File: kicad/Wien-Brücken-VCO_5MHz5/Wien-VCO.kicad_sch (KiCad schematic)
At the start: 22 parts, among them J1 J113, U1 ${SIM.NAME}

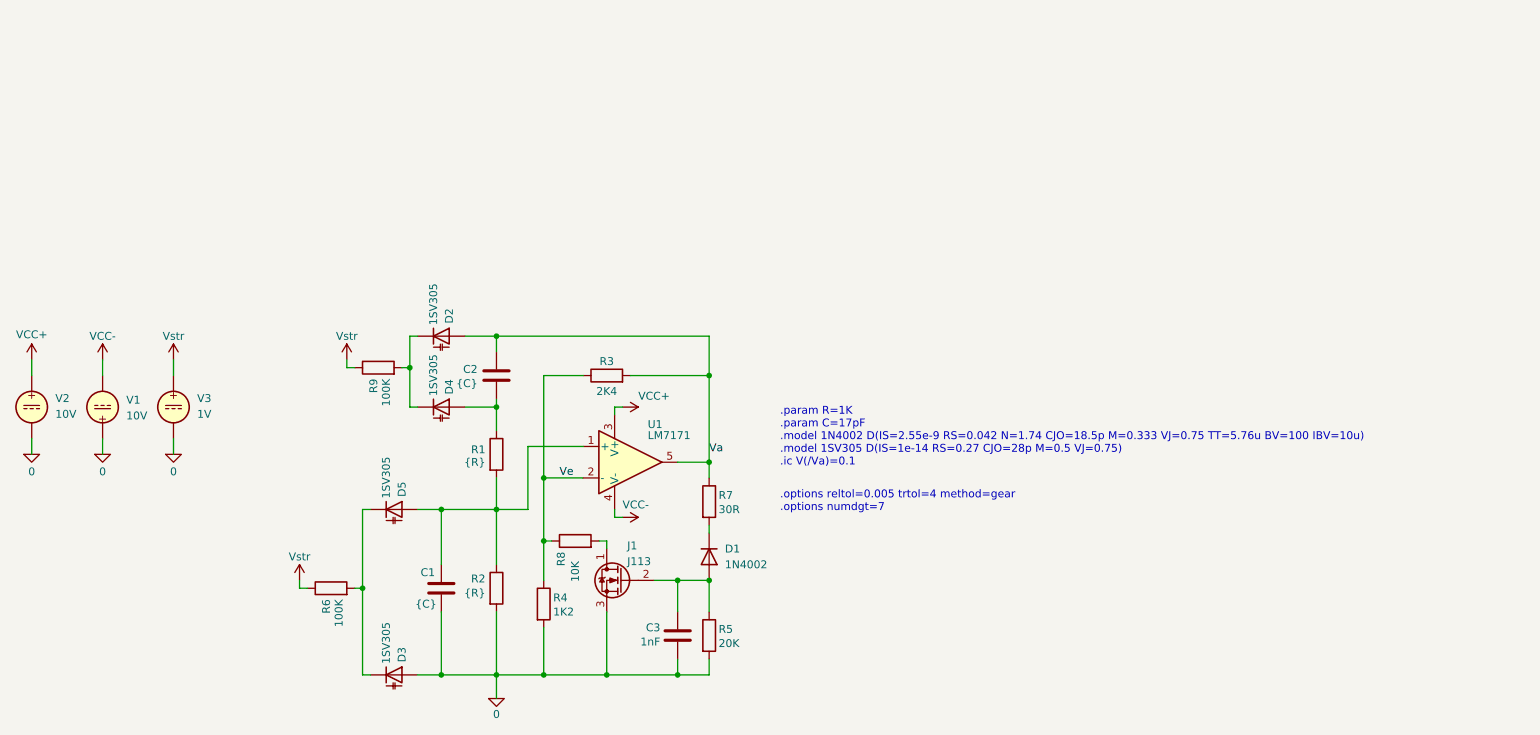
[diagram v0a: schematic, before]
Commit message: Erste Änderungen, Abgleiche LTspice vs ngspice
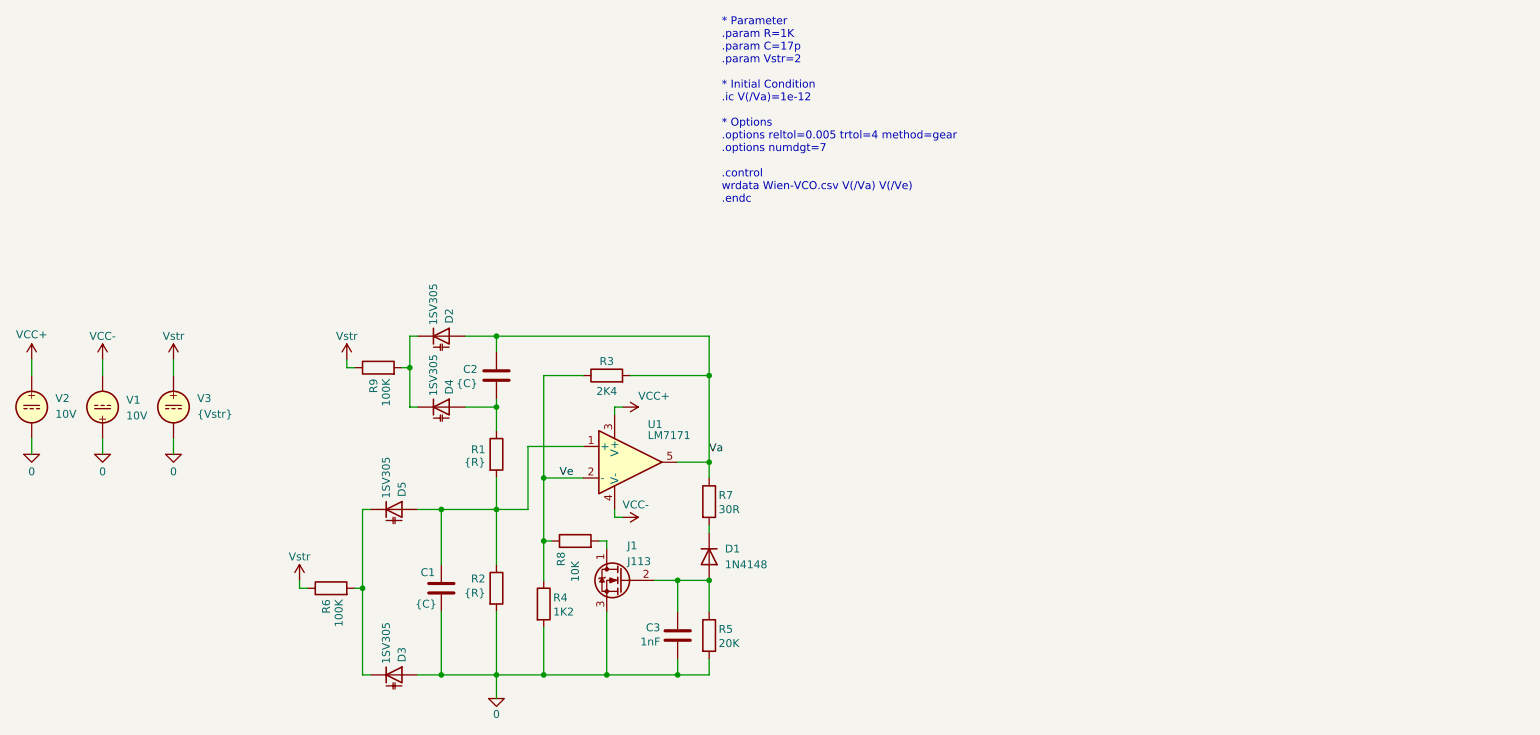
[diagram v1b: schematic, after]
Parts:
- D1: value 1N4002 -> 1N4148
- V3: value 1V -> {Vstr}
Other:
- note added: "* Parameter .param R=1K .param C=17p .param Vstr=2 * Initial Condition .ic V(/Va)=1e-12 * Options .options reltol=0.005 trtol=4 method=gear .options numdgt=7 .control wrdata Wien-VCO.csv V(/Va) V(/Ve) .endc"
- note removed: ".options reltol=0.005 trtol=4 method=gear .options numdgt=7"
- note removed: ".param R=1K .param C=17pF .model 1N4002 D(IS=2.55e-9 RS=0.042 N=1.74 CJO=18.5p M=0.333 VJ=0.75 TT=5.76u BV=100 IBV=10u) .model 1SV305 D(IS=1e-14 RS=0.27 CJO=28p M=0.5 VJ=0.75) .ic V(/Va)=0.1"
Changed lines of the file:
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@@
 	(generator_version "10.0")
 	(paper "A4")
-	(text ".param R=1K\n.param C=17pF\n.model 1N4002 D(IS=2.55e-9 RS=0.042 N=1.74 CJO=18.5p M=0.333 VJ=0.75 TT=5.76u BV=100 IBV=10u)\n.model 1SV305 D(IS=1e-14 RS=0.27 CJO=28p M=0.5 VJ=0.75)\n.ic V(/Va)=0.1"
+	(text "* Parameter\n.param R=1K\n.param C=17p\n.param Vstr=2\n\n* Initial Condition\n.ic V(/Va)=1e-12\n\n* Options\n.options reltol=0.005 trtol=4 method=gear\n.options numdgt=7\n\n.control\nwrdata Wien-VCO.csv V(/Va) V(/Ve)\n.endc"
 		(exclude_from_sim no)
-		(at 168.91 93.726 0)
+		(at 159.512 41.148 0)
 		(effects
 			(font
@@
 		)
 	)
-	(text ".options reltol=0.005 trtol=4 method=gear\n.options numdgt=7"
+	(text ""
 		(exclude_from_sim yes)
 		(at 168.91 104.14 0)
@@
 	)
 	(junction
-		(at 157.48 116.84)
+		(at 157.48 97.79)
 		(diameter 0)
 		(color 0 0 0 0)
 	)
 	(junction
-		(at 157.48 97.79)
+		(at 130.81 100.33)
 		(diameter 0)
 		(color 0 0 0 0)
 	)
 	(junction
-		(at 130.81 100.33)
+		(at 109.22 82.55)
 		(diameter 0)
 		(color 0 0 0 0)
 	)
 	(junction
-		(at 109.22 82.55)
+		(at 157.48 116.84)
 		(diameter 0)
 		(color 0 0 0 0)
@@
 			)
 		)
-		(property "Sim.Library" "..\\spicelibs\\lm7171.lib"
+		(property "Sim.Library" "../spicelibs/lm7171.lib"
 			(at 144.78 97.79 0)
 			(hide yes)
@@
 	)
 	(symbol
+		(lib_id "Diode:1N4148")
+		(at 157.48 113.03 270)
+		(unit 1)
+		(body_style 1)
+		(exclude_from_sim no)
+		(in_bom yes)
+		(on_board yes)
+		(in_pos_files yes)
+		(dnp no)
+		(fields_autoplaced yes)
+		(property "Reference" "D1"
+			(at 160.02 111.7599 90)
+			(show_name no)
+			(do_not_autoplace no)
+			(effects
+				(font
+					(size 1.27 1.27)
+				)
+				(justify left)
+			)
+		)
+		(property "Value" "1N4148"
+			(at 160.02 114.2999 90)
+			(show_name no)
+			(do_not_autoplace no)
+			(effects
+				(font
+					(size 1.27 1.27)
+				)
+				(justify left)
+			)
+		)
+		(property "Footprint" "Diode_THT:D_DO-35_SOD27_P7.62mm_Horizontal"
+			(at 157.48 113.03 0)
+			(hide yes)
+			(show_name no)
+			(do_not_autoplace no)
+			(effects
+				(font
+					(size 1.27 1.27)
+				)
+			)
+		)
+		(property "Datasheet" "https://assets.nexperia.com/documents/data-sheet/1N4148_1N4448.pdf"
+			(at 157.48 113.03 0)
+			(hide yes)
+			(show_name no)
+			(do_not_autoplace no)
+			(effects
+				(font
+					(size 1.27 1.27)
+				)
+			)
+		)
+		(property "Description" "100V 0.15A standard switching diode, DO-35"
+			(at 157.48 113.03 0)
+			(hide yes)
+			(show_name no)
+			(do_not_autoplace no)
+			(effects
+				(font
+					(size 1.27 1.27)
+				)
+			)
+		)
+		(property "Sim.Device" "D"
+			(at 157.48 113.03 0)
+			(hide yes)
+			(show_name no)
+			(do_not_autoplace no)
+			(effects
+				(font
+					(size 1.27 1.27)
+				)
+			)
+		)
+		(property "Sim.Pins" "1=K 2=A"
+			(at 157.48 113.03 0)
+			(hide yes)
+			(show_name no)
+			(do_not_autoplace no)
+			(effects
+				(font
+					(size 1.27 1.27)
+				)
+			)
+		)
+		(property "Sim.Library" "../spicelibs/elk.lib"
+			(at 157.48 113.03 0)
+			(hide yes)
+			(show_name no)
+			(do_not_autoplace no)
+			(effects
+				(font
+					(size 1.27 1.27)
+				)
+			)
+		)
+		(property "Sim.Name" "D1N4148"
+			(at 157.48 113.03 0)
+			(hide yes)
+			(show_name no)
+			(do_not_autoplace no)
+			(effects
+				(font
+					(size 1.27 1.27)
+				)
+			)
+		)
+		(pin "1"
+		)
+		(pin "2"
+		)
+		(instances
+			(project "Wien-VCO"
+				(path "/61a7698a-1c0d-4258-9661-7a52612acc47"
+					(reference "D1")
+					(unit 1)
+				)
+			)
+		)
+	)
+	(symbol
 		(lib_id "Device:R")
 		(at 123.19 96.52 0)
@@
 	)
 	(symbol
-		(lib_id "Diode:1N4148")
-		(at 157.48 113.03 270)
+		(lib_id "Device:D_Capacitance")
+		(at 114.3 88.9 0)
 		(unit 1)
 		(body_style 1)
@@
 		(in_pos_files yes)
 		(dnp no)
-		(fields_autoplaced yes)
-		(property "Reference" "D1"
-			(at 160.02 111.7599 90)
+		(property "Reference" "D4"
+			(at 115.57 86.868 90)
 			(show_name no)
 			(do_not_autoplace no)
@@
 			)
 		)
-		(property "Value" "1N4002"
-			(at 160.02 114.2999 90)
+		(property "Value" "1SV305"
+			(at 113.03 87.122 90)
 			(show_name no)
 			(do_not_autoplace no)
@@
 			)
 		)
-		(property "Footprint" "Diode_THT:D_DO-35_SOD27_P7.62mm_Horizontal"
-			(at 157.48 113.03 0)
-			(hide yes)
-			(show_name no)
-			(do_not_autoplace no)
-			(effects
-				(font
-					(size 1.27 1.27)
-				)
-			)
-		)
-		(property "Datasheet" "https://assets.nexperia.com/documents/data-sheet/1N4148_1N4448.pdf"
-			(at 157.48 113.03 0)
-			(hide yes)
-			(show_name no)
-			(do_not_autoplace no)
-			(effects
-				(font
-					(size 1.27 1.27)
-				)
-			)
-		)
-		(property "Description" "100V 0.15A standard switching diode, DO-35"
-			(at 157.48 113.03 0)
-			(hide yes)
-			(show_name no)
-			(do_not_autoplace no)
-			(effects
-				(font
-					(size 1.27 1.27)
-				)
-			)
-		)
-		(property "Sim.Device" "1N4002"
-			(at 157.48 113.03 0)
+		(property "Footprint" ""
+			(at 114.3 88.9 0)
 			(hide yes)
 			(show_name no)
@@
 			)
 		)
-		(property "Sim.Pins" "1=K 2=A"
-			(at 157.48 113.03 0)
+		(property "Datasheet" ""
+			(at 114.3 88.9 0)
 			(hide yes)
 			(show_name no)
@@
 			)
 		)
-		(pin "2"
-		)
-		(pin "1"
-		)
-		(instances
-			(project "Wien-VCO"
-				(path "/61a7698a-1c0d-4258-9661-7a52612acc47"
-					(reference "D1")
-					(unit 1)
-				)
-			)
-		)
-	)
-	(symbol
-		(lib_id "Device:D_Capacitance")
-		(at 114.3 88.9 0)
-		(unit 1)
-		(body_style 1)
-		(exclude_from_sim no)
-		(in_bom yes)
-		(on_board yes)
-		(in_pos_files yes)
-		(dnp no)
-		(property "Reference" "D4"
-			(at 115.57 86.868 90)
-			(show_name no)
-			(do_not_autoplace no)
-			(effects
-				(font
-					(size 1.27 1.27)
-				)
-				(justify left)
-			)
-		)
-		(property "Value" "1SV305"
-			(at 113.03 87.122 90)
-			(show_name no)
-			(do_not_autoplace no)
-			(effects
-				(font
-					(size 1.27 1.27)
-				)
-				(justify left)
-			)
-		)
-		(property "Footprint" ""
+		(property "Description" "Variable capacitance diode"
 			(at 114.3 88.9 0)
 			(hide yes)
@@
 			)
 		)
-		(property "Datasheet" ""
+		(property "Sim.Device" "D"
 			(at 114.3 88.9 0)
 			(hide yes)
@@
 			)
 		)
-		(property "Description" "Variable capacitance diode"
+		(property "Sim.Pins" "1=K 2=A"
 			(at 114.3 88.9 0)
 			(hide yes)
@@
 			)
 		)
-		(property "Sim.Device" "1SV305"
+		(property "Sim.Library" "../spicelibs/elk.lib"
 			(at 114.3 88.9 0)
 			(hide yes)
@@
 			)
 		)
-		(property "Sim.Pins" "1=K 2=A"
+		(property "Sim.Name" "1SV305"
 			(at 114.3 88.9 0)
 			(hide yes)
@@
 			)
 		)
-		(property "Sim.Device" "1SV305"
+		(property "Sim.Device" "D"
 			(at 114.3 77.47 0)
 			(hide yes)
@@
 			)
 		)
+		(property "Sim.Library" "../spicelibs/elk.lib"
+			(at 114.3 77.47 0)
+			(hide yes)
+			(show_name no)
+			(do_not_autoplace no)
+			(effects
+				(font
+					(size 1.27 1.27)
+				)
+			)
+		)
+		(property "Sim.Name" "1SV305"
+			(at 114.3 77.47 0)
+			(hide yes)
+			(show_name no)
+			(do_not_autoplace no)
+			(effects
+				(font
+					(size 1.27 1.27)
+				)
+			)
+		)
 		(pin "2"
 		)
@@
 			)
 		)
-		(property "Sim.Device" "1SV305"
+		(property "Sim.Device" "D"
 			(at 106.68 105.41 0)
 			(hide yes)
@@
 			)
 		)
+		(property "Sim.Library" "../spicelibs/elk.lib"
+			(at 106.68 105.41 0)
+			(hide yes)
+			(show_name no)
+			(do_not_autoplace no)
+			(effects
+				(font
+					(size 1.27 1.27)
+				)
+			)
+		)
+		(property "Sim.Name" "1SV305"
+			(at 106.68 105.41 0)
+			(hide yes)
+			(show_name no)
+			(do_not_autoplace no)
+			(effects
+				(font
+					(size 1.27 1.27)
+				)
+			)
+		)
 		(pin "2"
 		)
@@
 			)
 		)
-		(property "Sim.Library" "..\\spicelibs\\MeinJ113.lib"
+		(property "Sim.Library" "../spicelibs/J113.lib"
 			(at 143.51 116.84 0)
 			(hide yes)
@@
 			)
 		)
-		(property "Sim.Name" "MeinJ113"
+		(property "Sim.Name" "J113"
 			(at 143.51 116.84 0)
 			(hide yes)
@@
 			)
 		)
-		(property "Value" "1V"
+		(property "Value" "{Vstr}"
 			(at 74.93 90.0401 0)
 			(show_name no)
@@
 			)
 		)
-		(property "Sim.Device" "1SV305"
+		(property "Sim.Device" "D"
 			(at 106.68 132.08 0)
 			(hide yes)
@@
 			(at 106.68 132.08 0)
 			(hide yes)
+			(show_name no)
+			(do_not_autoplace no)
+			(effects
+				(font
+					(size 1.27 1.27)
+				)
+			)
+		)
+		(property "Sim.Library" "../spicelibs/elk.lib"
+			(at 106.68 132.08 0)
+			(hide yes)
+			(show_name no)
+			(do_not_autoplace no)
+			(effects
+				(font
+					(size 1.27 1.27)
+				)
+			)
+		)
+		(property "Sim.Name" "1SV305"
+			(at 106.68 132.08 0)
+			(hide yes)
